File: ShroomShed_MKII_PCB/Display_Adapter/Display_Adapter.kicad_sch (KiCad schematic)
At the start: 2 parts, among them J1 Display_Touch_SPI, J7 Display_Touch_SPI

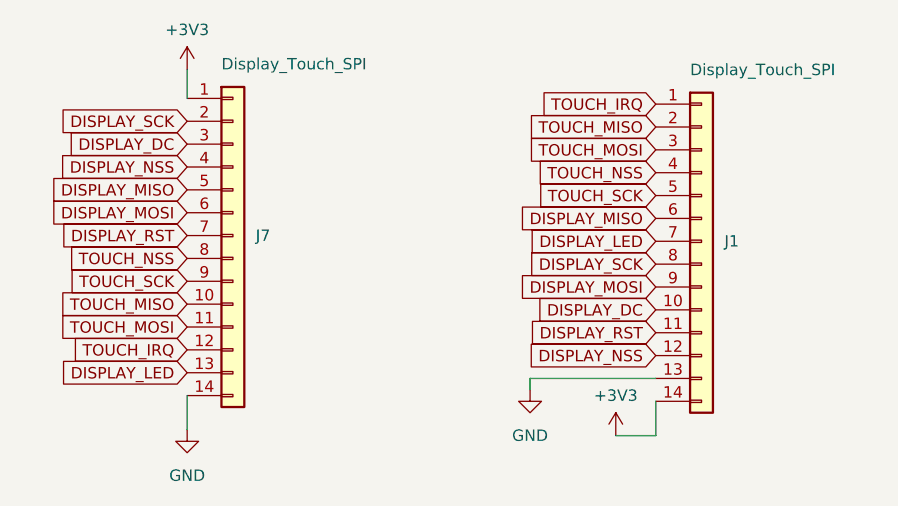
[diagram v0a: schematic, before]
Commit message: added solidworks files
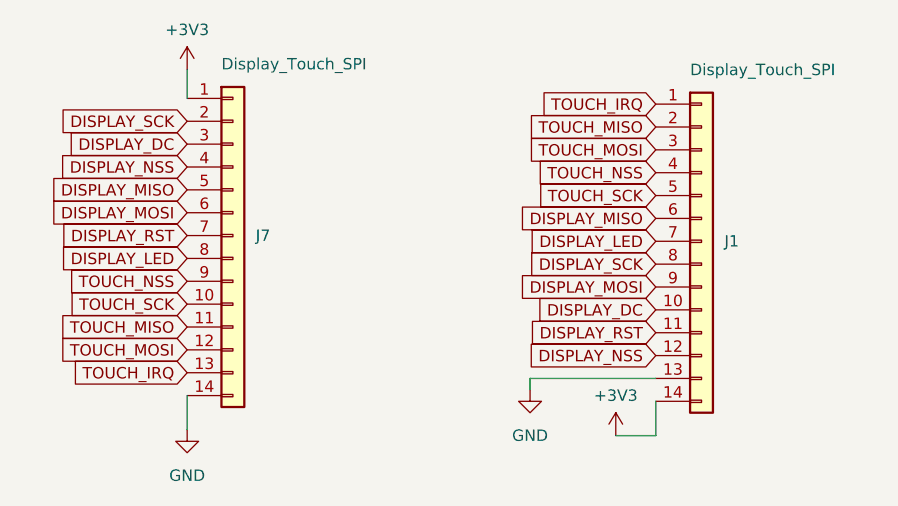
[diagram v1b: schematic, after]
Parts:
- J7: footprint DOWNLOAD_Connectors:CONN_532610001-SD_14_MOL -> DOWNLOAD_Connectors:MOLEX_530481410
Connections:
- net DISPLAY_LED: now also J7.8 (Pin_8); no longer J7.13 (Pin_13)
- net TOUCH_IRQ: now also J7.13 (Pin_13); no longer J7.12 (Pin_12)
- net TOUCH_MISO: now also J7.11 (Pin_11); no longer J7.10 (Pin_10)
- net TOUCH_MOSI: now also J7.12 (Pin_12); no longer J7.11 (Pin_11)
- net TOUCH_NSS: now also J7.9 (Pin_9); no longer J7.8 (Pin_8)
- net TOUCH_SCK: now also J7.10 (Pin_10); no longer J7.9 (Pin_9)
